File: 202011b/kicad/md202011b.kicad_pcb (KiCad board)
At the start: 2 copper layers, 83 x 79.4 mm, 48 parts, among them J101 MCU, J102 SocketA, J103 SocketB, J104 LED_EN, J201 ISP, Q101 MMBT3904, U101 STC15W104, U201 STC15W104

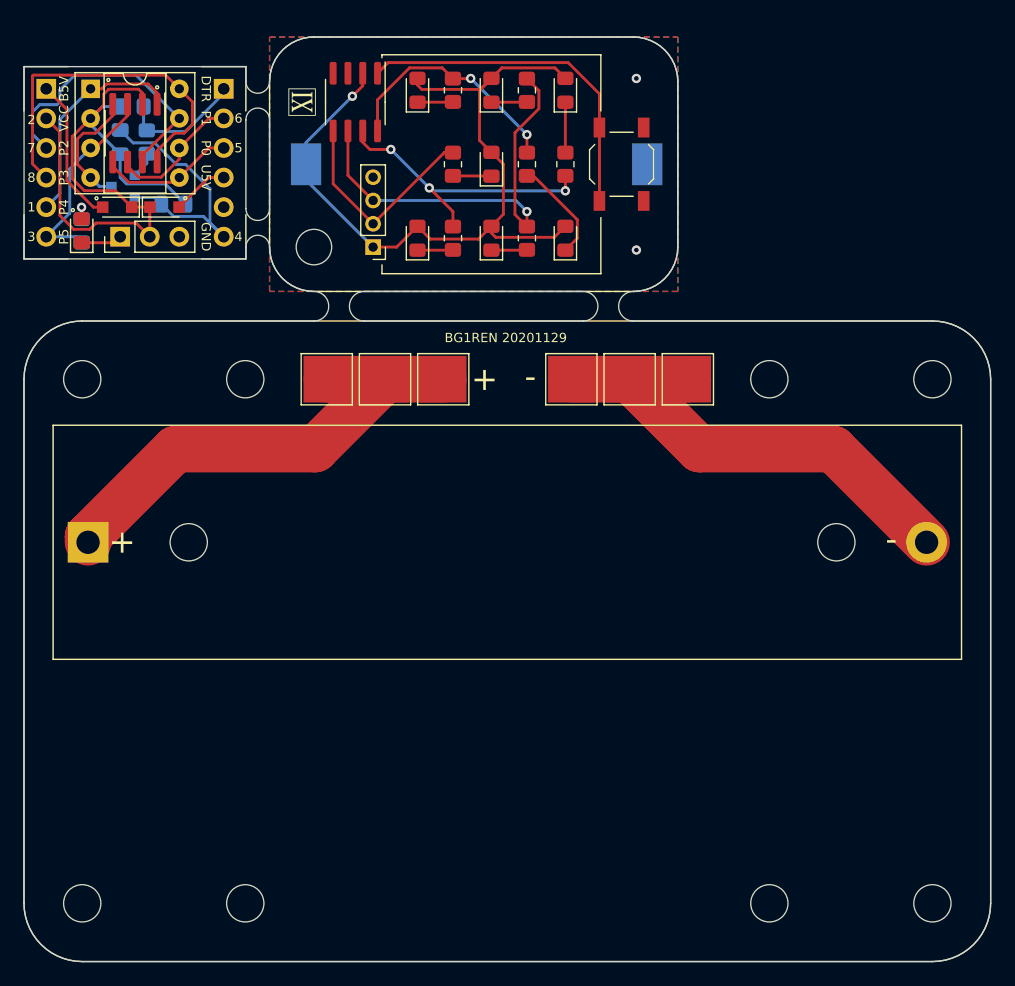
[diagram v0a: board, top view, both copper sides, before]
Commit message: Change PCB layout - 202011b-02
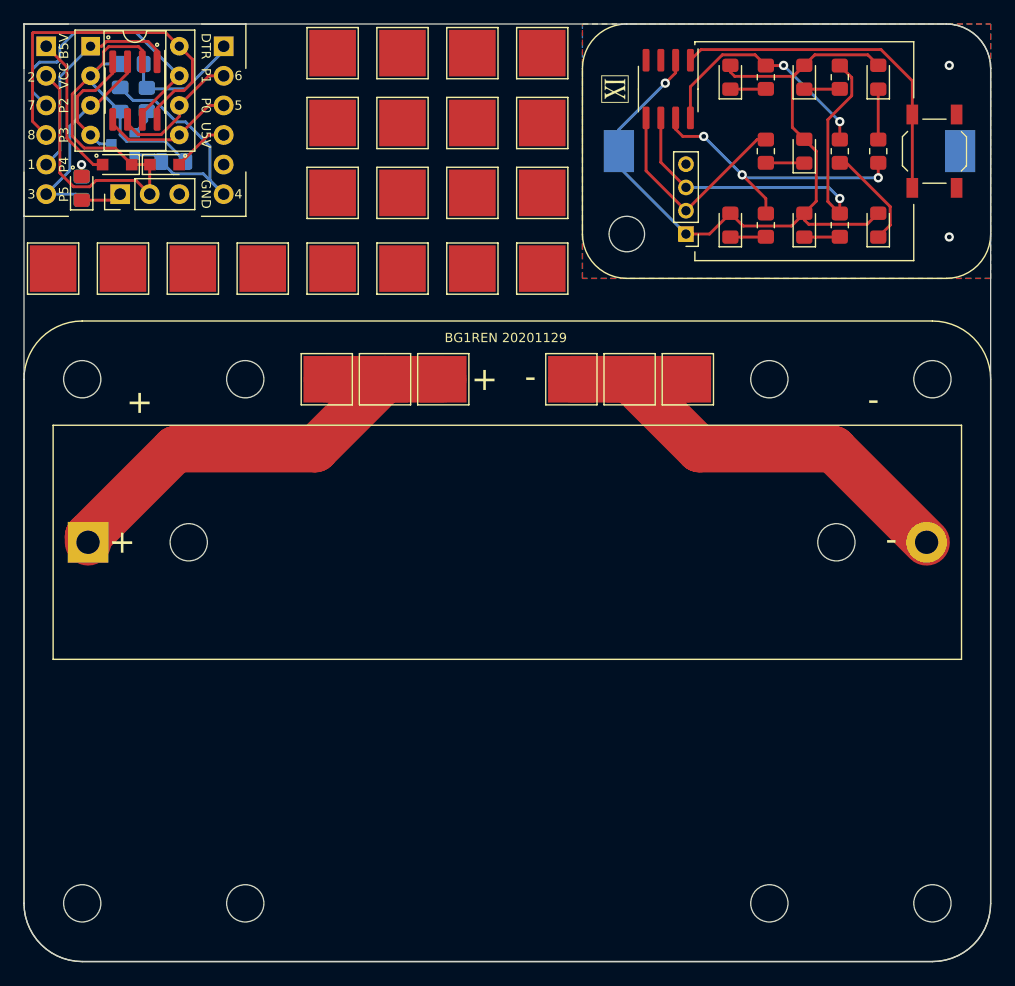
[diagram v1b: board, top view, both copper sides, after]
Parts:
- added REF**: TestPoint_Pad_4.0x4.0mm, TestPoint:TestPoint_Pad_4.0x4.0mm, F.Cu at (86.9, 73.6)
- added REF**: TestPoint_Pad_4.0x4.0mm, TestPoint:TestPoint_Pad_4.0x4.0mm, F.Cu at (92.9, 61.6)
- added REF**: TestPoint_Pad_4.0x4.0mm, TestPoint:TestPoint_Pad_4.0x4.0mm, F.Cu at (98.9, 61.6)
- added REF**: TestPoint_Pad_4.0x4.0mm, TestPoint:TestPoint_Pad_4.0x4.0mm, F.Cu at (104.9, 61.6)
- added REF**: TestPoint_Pad_4.0x4.0mm, TestPoint:TestPoint_Pad_4.0x4.0mm, F.Cu at (104.9, 80.1)
- added REF**: TestPoint_Pad_4.0x4.0mm, TestPoint:TestPoint_Pad_4.0x4.0mm, F.Cu at (98.9, 80.1)
- added REF**: TestPoint_Pad_4.0x4.0mm, TestPoint:TestPoint_Pad_4.0x4.0mm, F.Cu at (92.9, 80.1)
- added REF**: TestPoint_Pad_4.0x4.0mm, TestPoint:TestPoint_Pad_4.0x4.0mm, F.Cu at (86.9, 80.1)
- added REF**: TestPoint_Pad_4.0x4.0mm, TestPoint:TestPoint_Pad_4.0x4.0mm, F.Cu at (80.9, 80.1)
- added REF**: TestPoint_Pad_4.0x4.0mm, TestPoint:TestPoint_Pad_4.0x4.0mm, F.Cu at (74.9, 80.1)
- added REF**: TestPoint_Pad_4.0x4.0mm, TestPoint:TestPoint_Pad_4.0x4.0mm, F.Cu at (68.9, 80.1)
- added REF**: TestPoint_Pad_4.0x4.0mm, TestPoint:TestPoint_Pad_4.0x4.0mm, F.Cu at (92.9, 73.6)
- added REF**: TestPoint_Pad_4.0x4.0mm, TestPoint:TestPoint_Pad_4.0x4.0mm, F.Cu at (62.9, 80.1)
- added REF**: TestPoint_Pad_4.0x4.0mm, TestPoint:TestPoint_Pad_4.0x4.0mm, F.Cu at (98.9, 73.6)
- added REF**: TestPoint_Pad_4.0x4.0mm, TestPoint:TestPoint_Pad_4.0x4.0mm, F.Cu at (104.9, 73.6)
- added REF**: TestPoint_Pad_4.0x4.0mm, TestPoint:TestPoint_Pad_4.0x4.0mm, F.Cu at (86.9, 67.6)
- added REF**: TestPoint_Pad_4.0x4.0mm, TestPoint:TestPoint_Pad_4.0x4.0mm, F.Cu at (92.9, 67.6)
- added REF**: TestPoint_Pad_4.0x4.0mm, TestPoint:TestPoint_Pad_4.0x4.0mm, F.Cu at (98.9, 67.6)
- added REF**: TestPoint_Pad_4.0x4.0mm, TestPoint:TestPoint_Pad_4.0x4.0mm, F.Cu at (104.9, 67.6)
- added REF**: TestPoint_Pad_4.0x4.0mm, TestPoint:TestPoint_Pad_4.0x4.0mm, F.Cu at (86.9, 61.6)
- moved D201 26.9 mm to (127.4, 70.0)
- moved D202 26.9 mm to (127.4, 76.4)
- moved D203 26.9 mm to (127.4, 63.7)
- moved D204 26.9 mm to (121.1, 76.4)
- moved D206 26.9 mm to (121.1, 63.7)
- moved G*** 26.9 mm to (111.2, 64.7)
- moved R201 26.9 mm to (124.1, 70.0)
- moved R204 26.9 mm to (124.1, 76.4)
- moved R206 26.9 mm to (124.1, 63.7)
- moved SW_201 26.9 mm to (138.6, 70.0)
- moved BT201 26.9 mm to (126.2, 70.0)
- moved D205 26.9 mm to (133.8, 63.7)
- moved D207 26.9 mm to (133.8, 76.4)
- moved J201 26.9 mm to (117.3, 77.1)
- moved R202 26.9 mm to (130.5, 76.4)
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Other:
- board size 83 x 79.4 mm -> 83 x 80.5 mm
